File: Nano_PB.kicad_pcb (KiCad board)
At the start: 2 copper layers, 100 x 40 mm, 97 parts, among them CON1 BARREL_JACK, P1 CONN_01X06, P2 CONN_01X01, P3 CONN_01X03, P4 CONN_01X03, P5 CONN_01X03, P6 CONN_01X04, Q1 SMBT3904, Q10 BSS138, Q2 SMBT3904, Q3 SMBT3904, Q4 SMBT3904, Q5 SMBT3904, Q6 BC846B, Q7 BC846B, Q8 BC846B, Q9 BSS138, SW1 Izquierda, SW2 Arriba, SW3 Abajo, SW4 Derecha, U1 Arduino_Nano, U2 LM7805CT, U3 Matriz_5x7, U4 74HC595, U5 74HC595, U6 74HC148, U7 MMA7660FC

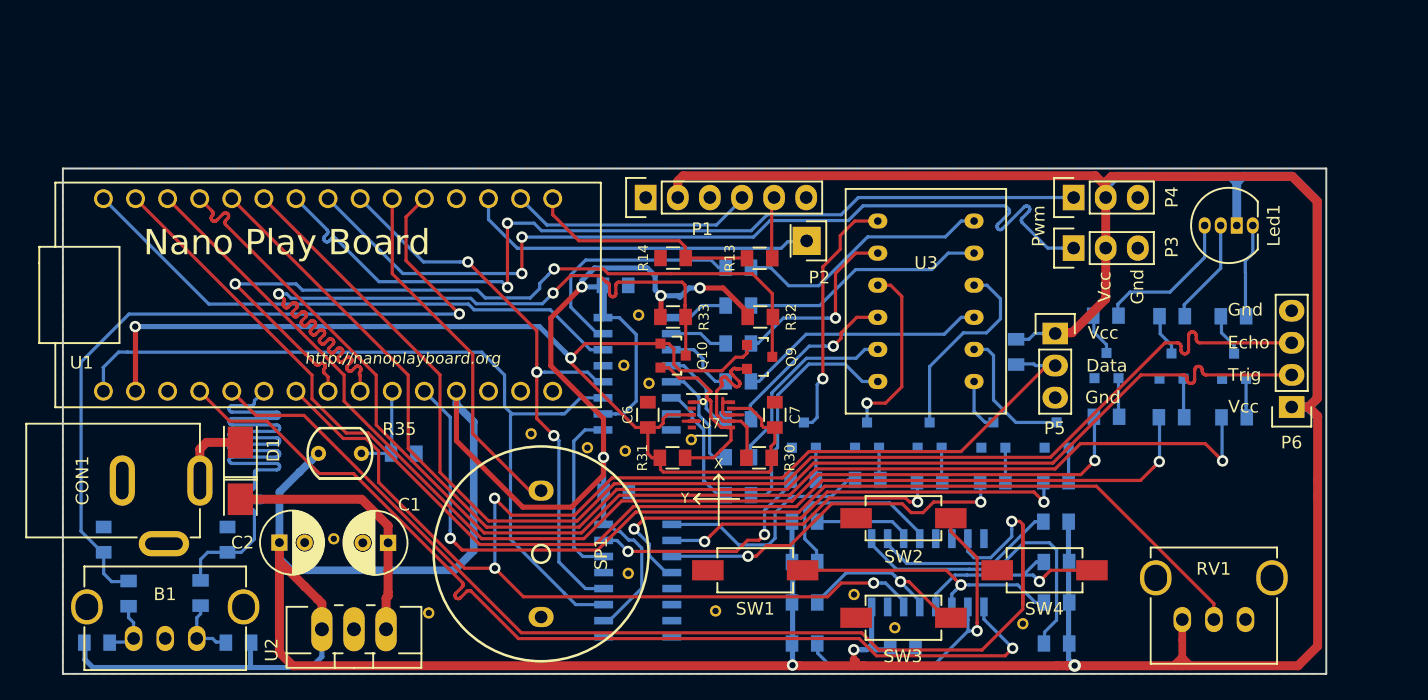
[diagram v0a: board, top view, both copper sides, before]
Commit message: finalizado enrutado provisional
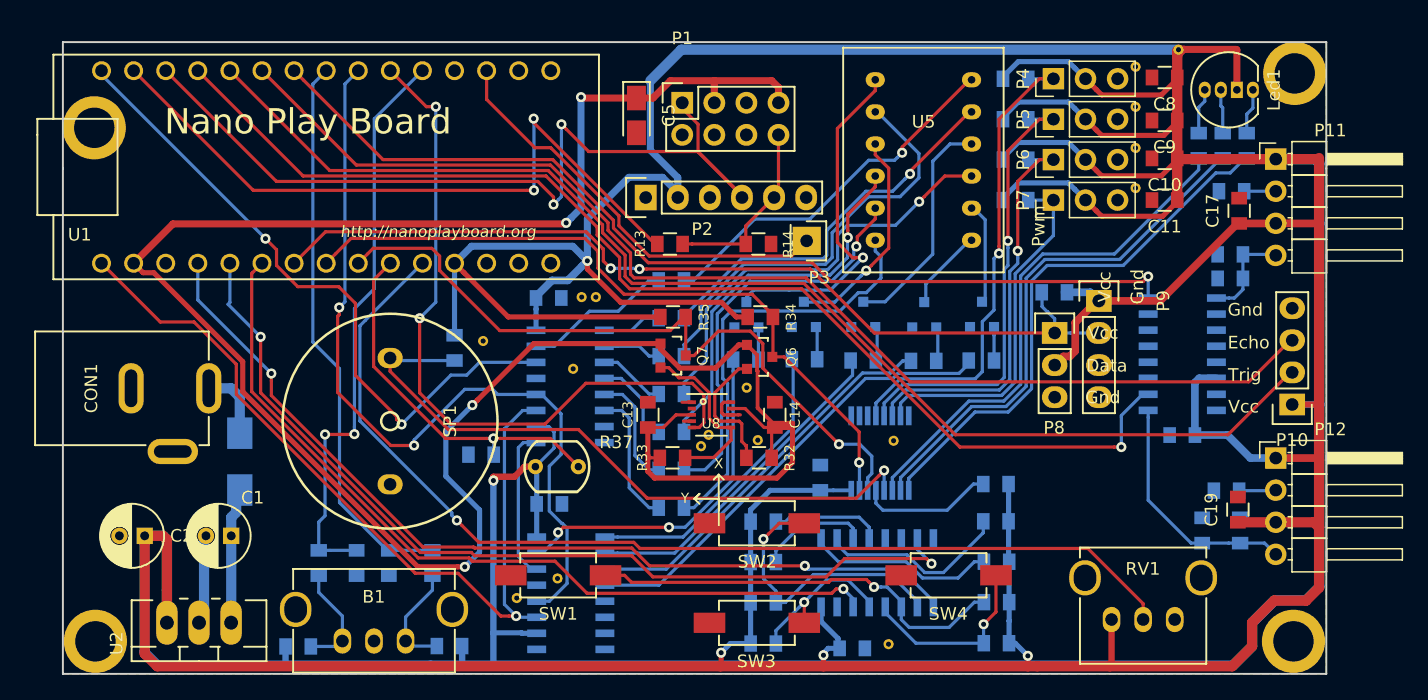
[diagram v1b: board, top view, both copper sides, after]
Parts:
- removed G***: LOGO, logos:osh-logo
- removed G***: LOGO, logos:logo_HackLabAl
- removed the Gnd-Via at (101.8, 56.2)
- removed the Gnd-Via at (93.6, 56.9)
- removed the Gnd-Via at (103.8, 69.8)
- removed the Gnd-Via at (114.7, 68.5)
- removed the Gnd-Via at (96.5, 50.4)
- removed the Gnd-Via at (128.1, 70.8)
- removed the Gnd-Via at (81.0, 70.0)
- removed the Gnd-Via at (117.9, 71.1)
- removed the Gnd-Via at (97.7, 46.4)
- removed the Gnd-Via at (98.5, 51.8)
- removed the Gnd-Via at (73.5, 64.1)
- removed the Gnd-Via at (96.6, 57.1)
- removed the Gnd-Via at (96.8, 66.8)
- removed the Gnd-Via at (89.2, 55.8)
- removed the P3 at (132.1, 41.1)
- removed the Q6 at (144.8, 50.4)
- removed the Q7 at (134.7, 50.4)
- removed Q8: BC846B, TO_SOT_Packages_SMD:SOT-23
- added C10: 1u, Capacitors_SMD:C_0805, F.Cu at (139.3, 34.0)
- added C11: 1u, Capacitors_SMD:C_0805, F.Cu at (139.3, 37.3)
- added C17: 100n, Capacitors_SMD:C_0805, F.Cu at (145.2, 38.1)
- added C18: 10n, Capacitors_SMD:C_0805, B.Cu at (144.5, 43.5)
- added C19: 100n, Capacitors_SMD:C_0805, F.Cu at (145.1, 61.8)
- added C20: 10n, Capacitors_SMD:C_0805, B.Cu at (142.3, 63.4)
- added C21: 100n, Capacitors_SMD:C_0805, B.Cu at (140.7, 55.9)
- added C5: 10u, Capacitors_Tantalum_SMD:Tantalum_Case-A_EIA-3216-18_Reflow, F.Cu at (97.5, 30.6)
- added C7: 100n, Capacitors_SMD:C_0805, B.Cu at (112.0, 59.2)
- added C8: 1u, Capacitors_SMD:C_0805, F.Cu at (139.3, 27.6)
- added C9: 1u, Capacitors_SMD:C_0805, F.Cu at (139.3, 31.0)
- added Gnd-Via: VAL**, Vias:Gnd-Via, F.Cu at (54.6, 31.6)
- added Gnd-Via: VAL**, Vias:Gnd-Via, F.Cu at (54.7, 72.2)
- added Gnd-Via: VAL**, Vias:Gnd-Via, F.Cu at (149.5, 72.2)
- added Gnd-Via: VAL**, Vias:Gnd-Via, F.Cu at (117.4, 72.4)
- added Gnd-Via: VAL**, Vias:Gnd-Via, F.Cu at (88.0, 68.8)
- added Gnd-Via: VAL**, Vias:Gnd-Via, F.Cu at (91.2, 67.2)
- added Gnd-Via: VAL**, Vias:Gnd-Via, F.Cu at (107.1, 56.3)
- added Gnd-Via: VAL**, Vias:Gnd-Via, F.Cu at (103.2, 55.9)
- added Gnd-Via: VAL**, Vias:Gnd-Via, F.Cu at (137.0, 26.7)
- added Gnd-Via: VAL**, Vias:Gnd-Via, F.Cu at (137.0, 29.9)
- added Gnd-Via: VAL**, Vias:Gnd-Via, F.Cu at (137.0, 33.1)
- added Gnd-Via: VAL**, Vias:Gnd-Via, F.Cu at (85.3, 48.4)
- added Gnd-Via: VAL**, Vias:Gnd-Via, F.Cu at (137.0, 36.3)
- added Gnd-Via: VAL**, Vias:Gnd-Via, F.Cu at (106.2, 52.1)
- added Gnd-Via: VAL**, Vias:Gnd-Via, F.Cu at (102.6, 56.8)
- added Gnd-Via: VAL**, Vias:Gnd-Via, F.Cu at (92.5, 50.6)
- added Gnd-Via: VAL**, Vias:Gnd-Via, F.Cu at (94.3, 45.0)
- added Gnd-Via: VAL**, Vias:Gnd-Via, F.Cu at (93.2, 45.0)
- added Gnd-Via: VAL**, Vias:Gnd-Via, F.Cu at (117.8, 56.3)
- added Gnd-Via: VAL**, Vias:Gnd-Via, F.Cu at (140.4, 25.4)
- added Gnd-Via: VAL**, Vias:Gnd-Via, F.Cu at (149.6, 27.2)
- added P1: CONN_02X04, Socket_Strips:Socket_Strip_Straight_2x04, F.Cu at (101.1, 29.6)
- added P11: CONN_01X04, Pin_Headers:Pin_Header_Angled_1x04_Pitch2.54mm, F.Cu at (148.1, 34.0)
- added P12: CONN_01X04, Pin_Headers:Pin_Header_Angled_1x04_Pitch2.54mm, F.Cu at (148.1, 57.7)
- added P5: CONN_01X03, Pin_Headers:Pin_Header_Straight_1x03_Pitch2.54mm, F.Cu at (130.5, 30.9)
- added P6: CONN_01X03, Pin_Headers:Pin_Header_Straight_1x03_Pitch2.54mm, F.Cu at (130.5, 34.1)
- added P7: CONN_01X03, Pin_Headers:Pin_Header_Straight_1x03_Pitch2.54mm, F.Cu at (130.5, 37.3)
- added P9: CONN_01X04, Socket_Strips:Socket_Strip_Straight_1x04, F.Cu at (134.1, 45.2)
- added R21: 120, Resistencias:R_0805, B.Cu at (142.0, 33.0)
- added R22: 120, Resistencias:R_0805, B.Cu at (143.9, 33.0)
- added R36: 10K, Resistencias:R_0805, B.Cu at (83.1, 49.0)
- added R43: 220R, Resistencias:R_0805, B.Cu at (144.6, 36.6)
- added R44: 47K, Resistencias:R_0805, B.Cu at (144.5, 41.6)
- added R45: 220R, Resistencias:R_0805, B.Cu at (144.2, 60.3)
- added R46: 47K, Resistencias:R_0805, B.Cu at (145.3, 63.4)
- added U6: PCA9551, Housings_SSOP:TSSOP-16_4.4x5mm_Pitch0.65mm, B.Cu at (116.8, 57.3)
- added U9: 40106, Housings_SOIC:SOIC-16_3.9x9.9mm_Pitch1.27mm, B.Cu at (140.7, 49.5)
- D1: moved to B.Cu
- P4: footprint Pin_Headers:Pin_Header_Straight_1x03 -> Pin_Headers:Pin_Header_Straight_1x03_Pitch2.54mm
- R15, R16, R17: value 4K7 -> 10K
- R18, R19: value 100 -> 10K
- R20: value 100 -> 120
- moved R16 27.7 mm to (127.5, 27.7), turned to 0 degrees
- moved R17 26.6 mm to (127.5, 30.9), turned to 0 degrees
- moved R18 21.2 mm to (127.5, 34.1), turned to 0 degrees
- moved C15 20.1 mm to (75.3, 66.0), turned to 270 degrees
- moved R15 19.6 mm to (125.9, 59.7)
- moved R42 18.5 mm to (81.3, 66.0)
- moved R37 17.2 mm to (91.2, 58.4)
- moved R41 16.7 mm to (82.7, 72.6)
- moved B1 16.5 mm to (76.7, 72.2)
- moved R39 15.9 mm to (70.7, 72.6)
- moved SP1 15.9 mm to (78.0, 54.8)
- moved SW1 15.6 mm to (91.3, 67.0)
- moved R40 15.2 mm to (72.3, 66.0)
- moved R20 14.7 mm to (145.8, 33.0), turned to 270 degrees
- moved C16 12.9 mm to (77.9, 66.0), turned to 270 degrees
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- renumbered C5 to C12, C6 to C13, C7 to C14, C8 to C15, C9 to C16, P6 to P10, P1 to P2, P2 to P3, P5 to P8, Q9 to Q6, Q10 to Q7, R21 to R23, R22 to R24, R26 to R25, R23 to R26, R24 to R28, R28 to R29, R25 to R30, R29 to R31, R30 to R32, R31 to R33, R32 to R34, R33 to R35, R35 to R37, R36 to R38, R37 to R39, R38 to R40, R39 to R41, R40 to R42, U4 to U3, U5 to U4, U3 to U5, U6 to U7, U7 to U8
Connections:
- C16 pad 1: A2 -> D5
- P2 pad 4: D0 -> D10
- P2 pad 5: Net-(P1-Pad5) -> /Bluetooth/RxD
- P4 pad 1: D6 -> SERVO1
- P8 pad 1: +5V -> A3
- P8 pad 2: A3 -> +5V
- R13 pad 1: Net-(P1-Pad5) -> /Bluetooth/RxD
- R13 pad 2: D1 -> D11
- R14 pad 1: D1 -> /Bluetooth/RxD
- R15 pad 1: Net-(Q6-Pad1) -> +5V
- R15 pad 2: D9 -> Net-(R15-Pad2)
- R16 pad 1: Net-(Q7-Pad1) -> +5V
- R16 pad 2: D10 -> SERVO1
- R17 pad 1: Net-(Q8-Pad1) -> +5V
- R17 pad 2: D11 -> SERVO2
- R18 pad 1: Net-(Led1-Pad4) -> +5V
- R18 pad 2: Net-(Q6-Pad3) -> SERVO3
- R19 pad 1: Net-(Led1-Pad1) -> +5V
- R19 pad 2: Net-(Q7-Pad3) -> SERVO4
- R20 pad 1: Net-(Led1-Pad2) -> Net-(Led1-Pad4)
- R20 pad 2: Net-(Q8-Pad3) -> LED_RED
- R42 pad 2: A2 -> D5
- SP1 pad 1: D3 -> BUZZER
- U1 pad 1: D1 -> Net-(U1-Pad1)
- U1 pad 2: D0 -> Net-(U1-Pad2)
- U7 pad 14: A3 -> A2
- U8 pad 5: Net-(U7-Pad5) -> D3
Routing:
- net +5V: track 479.9 -> 669.6 mm, vias 7 -> 5
- net +3V3: track 91.5 -> 184.2 mm, vias 2 -> 4
- net BUZZER: track 0.00 -> 52.0 mm, vias 0 -> 1
- net D11: track 99.7 -> 55.4 mm, vias 1 -> 2
- net A3: track 116.6 -> 72.4 mm, vias 3 -> 2
- net LED_RED: track 0.00 -> 43.2 mm
- net LED_BLUE: track 0.00 -> 42.0 mm
- net LED_GREEN: track 0.00 -> 41.3 mm
- net SERVO1: track 0.00 -> 38.6 mm, vias 0 -> 1
- net SERVO2: track 0.00 -> 36.0 mm, vias 0 -> 1
- net SERVO3: track 0.00 -> 32.6 mm, vias 0 -> 1
- net SERVO4: track 0.00 -> 28.4 mm
- net D3: track 28.5 -> 56.5 mm, vias 0 -> 2
- net D5: track 72.0 -> 44.4 mm, vias 2 -> 0
- net D10: track 91.8 -> 68.1 mm, vias 1 -> 2
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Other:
- board size 100 x 40 mm -> 100 x 50 mm
- net class Default: via_dia 0.9 -> 0.8; via_drill 0.5 -> 0.4
- net class Power: via_dia 1 -> 0.8; via_drill 0.5 -> 0.4
